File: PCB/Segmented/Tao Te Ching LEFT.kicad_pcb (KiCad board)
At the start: 2 copper layers, 138.1 x 92.9 mm, 49 parts, among them SW1 SW_Push_45deg, SW10 SW_Push_45deg, SW11 SW_Push_45deg, SW12 SW_Push_45deg, SW13 SW_Push_45deg, SW14 SW_Push_45deg, SW15 SW_Push_45deg, SW16 SW_Push_45deg, SW17 SW_Push_45deg, SW18 SW_Push_45deg, SW19 SW_Push_45deg, SW2 SW_Push_45deg, SW20 SW_Push_45deg, SW21 SW_Push_45deg, SW22 SW_Push_45deg, SW23 SW_Push_45deg, SW24 SW_Push_45deg, SW3 SW_Push_45deg, SW4 SW_Push_45deg, SW5 SW_Push_45deg, SW6 SW_Push_45deg, SW7 SW_Push_45deg, SW8 SW_Push_45deg, SW9 SW_Push_45deg, U1 XIAO-nRF52840-DIP

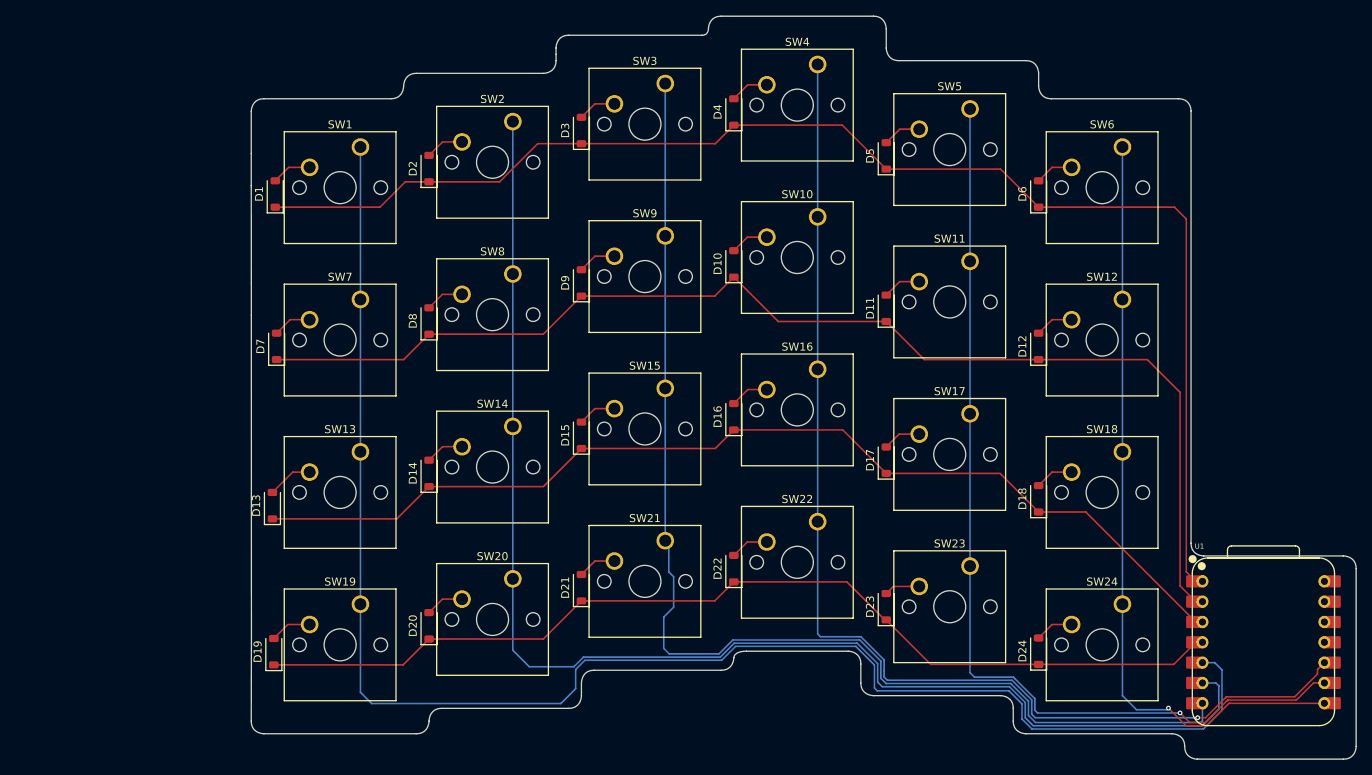
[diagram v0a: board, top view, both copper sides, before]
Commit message: Reworked Case and images
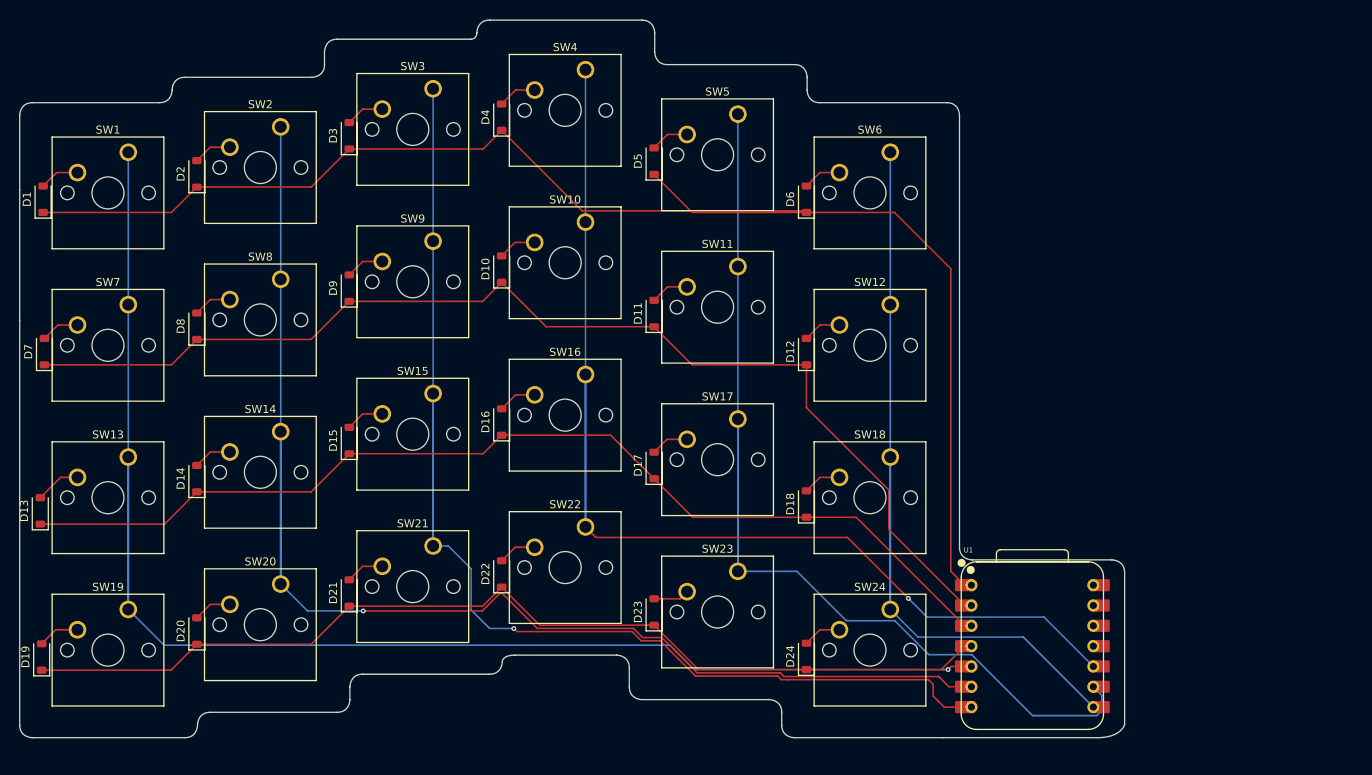
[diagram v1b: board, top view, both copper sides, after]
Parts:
- moved D10 29.0 mm to (181.3, 76.7)
- moved D12 29.0 mm to (219.4, 87.1)
- moved D14 29.0 mm to (143.2, 102.9)
- moved D15 29.0 mm to (162.2, 98.2)
- moved D16 29.0 mm to (181.3, 95.9)
- moved D18 29.0 mm to (219.4, 106.1)
- moved D19 29.0 mm to (123.8, 125.2)
- moved D2 29.0 mm to (143.2, 64.8)
- moved D20 29.0 mm to (143.2, 122.0)
- moved D21 29.0 mm to (162.2, 117.2)
- moved D22 29.0 mm to (181.3, 114.8)
- moved D24 29.0 mm to (219.4, 125.2)
- moved D3 29.0 mm to (162.2, 60.1)
- moved D4 29.0 mm to (181.3, 57.8)
- moved D6 29.0 mm to (219.4, 68.0)
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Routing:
- net Row0: track 168.8 -> 187.0 mm
- net Col4: track 120.3 -> 133.7 mm, vias 1 -> 0
- net Col0: track 196.7 -> 185.7 mm, vias 0 -> 1
- net Col5: track 96.7 -> 107.5 mm, vias 1 -> 0
- net Row1: track 150.2 -> 142.9 mm
- net Col2: track 148.8 -> 155.7 mm, vias 0 -> 1
- net Col3: track 144.4 -> 147.7 mm
- net Col1: track 169.1 -> 170.5 mm, vias 0 -> 1
- net Row3: track 125.0 -> 126.0 mm
- net Row2: track 130.0 -> 130.9 mm
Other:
- board size 138.1 x 92.9 mm -> 138.1 x 89.7 mm
